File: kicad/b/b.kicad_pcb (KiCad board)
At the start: 2 copper layers, 75 x 40 mm, 12 parts, among them J1 Conn_01x01_Socket, J2 Conn_01x01_Socket, J3 Conn_01x01_Socket, J4 Conn_01x01_Socket, J5 Conn_01x01_Socket, J6 Conn_01x01_Socket, U1 ABX00012

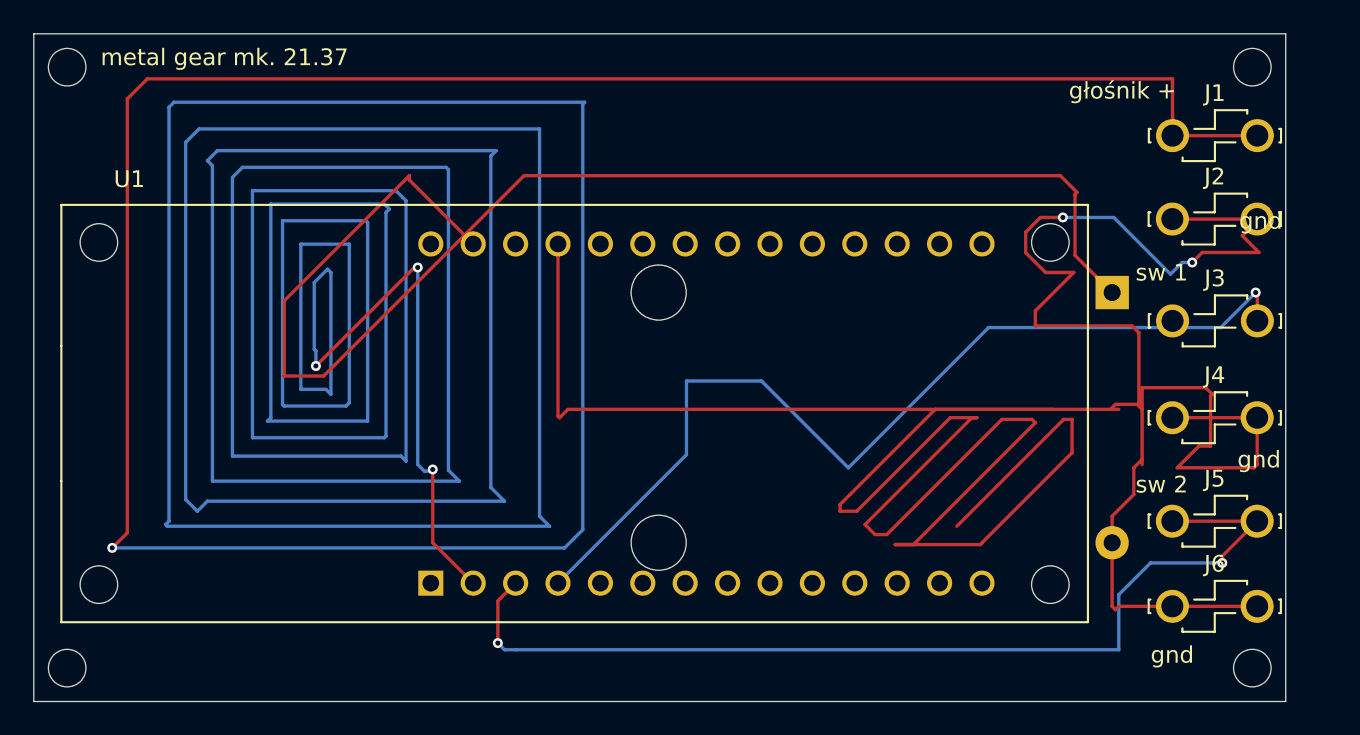
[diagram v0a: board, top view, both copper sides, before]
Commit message: kicad done
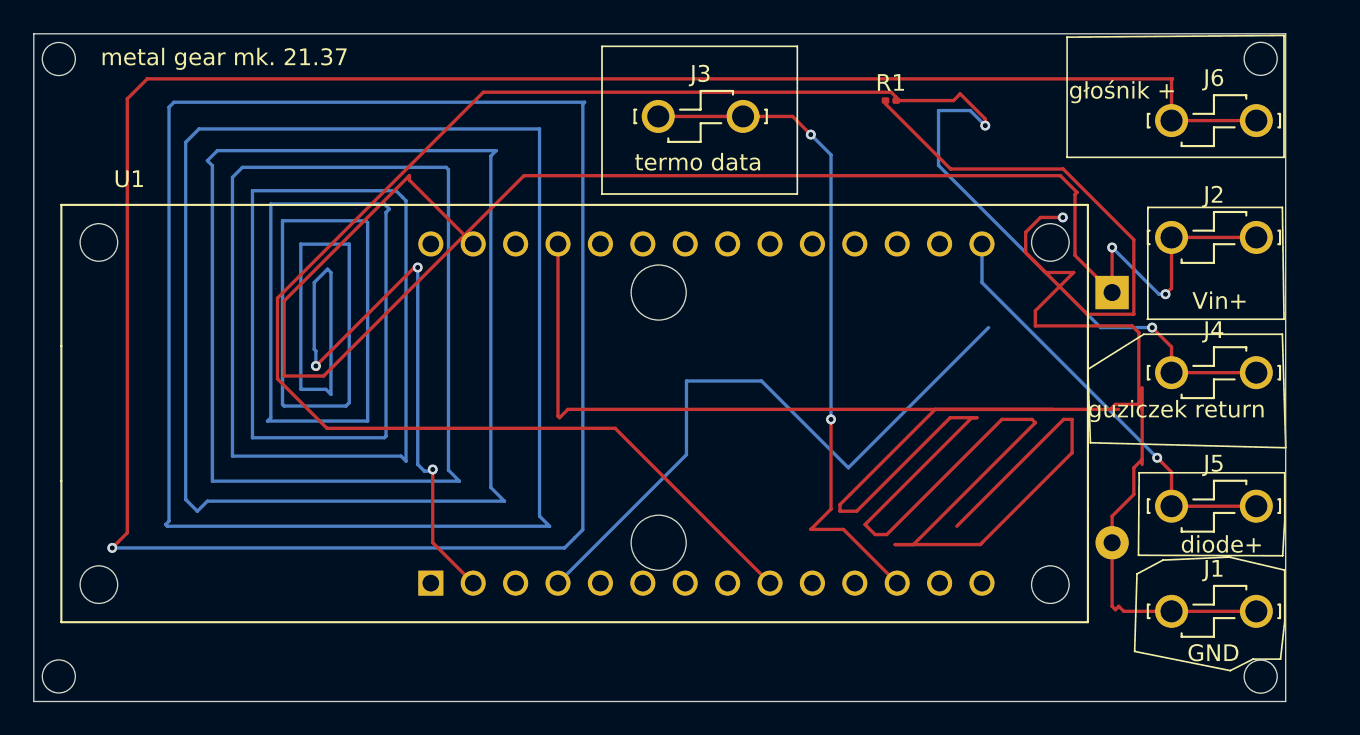
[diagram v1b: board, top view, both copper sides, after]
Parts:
- removed ? (x4): , 
- added R1: 10000, Resistor_SMD:R_0201_0603Metric, F.Cu at (241.3, 109.0)
- moved J3 33.2 mm to (229.9, 110.0)
- moved J6 29.1 mm to (260.7, 110.2)
- moved J1 28.5 mm to (260.7, 139.6)
- moved J4 2.70 mm to (260.7, 125.3)
- moved J2 1.10 mm to (260.7, 117.2)
- moved J5 0.90 mm to (260.7, 133.3)
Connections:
- J1 pad 1_1: Net-(J6-Pin_1) -> GND
- J1 pad 1_2: Net-(J6-Pin_1) -> GND
- J2 pad 1_1: GND -> Net-(BT1-+)
- J2 pad 1_2: GND -> Net-(BT1-+)
- J3 pad 1_1: Net-(J4-Pin_1) -> Net-(J3-Pin_1)
- J3 pad 1_2: Net-(J4-Pin_1) -> Net-(J3-Pin_1)
- J4 pad 1_1: GND -> Net-(J4-Pin_1)
- J4 pad 1_2: GND -> Net-(J4-Pin_1)
- J5 pad 1_1: Net-(J3-Pin_1) -> Net-(J5-Pin_1)
- J5 pad 1_2: Net-(J3-Pin_1) -> Net-(J5-Pin_1)
- J6 pad 1_1: GND -> Net-(J6-Pin_1)
- J6 pad 1_2: GND -> Net-(J6-Pin_1)
- U1 pad 12: unconnected-(U1-PA11_TCC0-W3/~3-Pad12) -> Net-(J3-Pin_1)
- U1 pad 15: unconnected-(U1-PA20_TCC0-W6-Pad15) -> Net-(J5-Pin_1)
- U1 pad 3: Net-(J3-Pin_1) -> unconnected-(U1-PB02_AIN10/A1-Pad3)
- U1 pad 4: Net-(J4-Pin_1) -> unconnected-(U1-PB03_AIN11/A2-Pad4)
- U1 pad 9: unconnected-(U1-PA22_TC4-W0/0-Pad9) -> Net-(J4-Pin_1)
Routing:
- net Net-(J4-Pin_1): track 57.6 -> 120.0 mm, vias 1 -> 2
- net unconnected-(U1-PB03_AIN11/A2-Pad4): track 0.00 -> 39.0 mm
- net Net-(J5-Pin_1): track 0.00 -> 25.5 mm, vias 0 -> 1
- net Net-(J3-Pin_1): track 60.1 -> 40.8 mm
- net Net-(BT1-+): track 80.6 -> 96.3 mm, vias 0 -> 2
- net GND: track 220.3 -> 206.9 mm, vias 2 -> 1
- net Net-(J6-Pin_1): track 632.1 -> 631.2 mm
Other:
- outline, holes or cut-outs redrawn
- board text added: "GND"
- board text added: "Vin+"
- board text added: "diode+"
- board text added: "guziczek return"
- board text added: "termo data"
- board text removed: "gnd"
- board text removed: "sw 1"
- board text removed: "sw 2"
